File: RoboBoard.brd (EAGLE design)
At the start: 66 x 78.4 mm, 31 parts, among them IC2 L293D

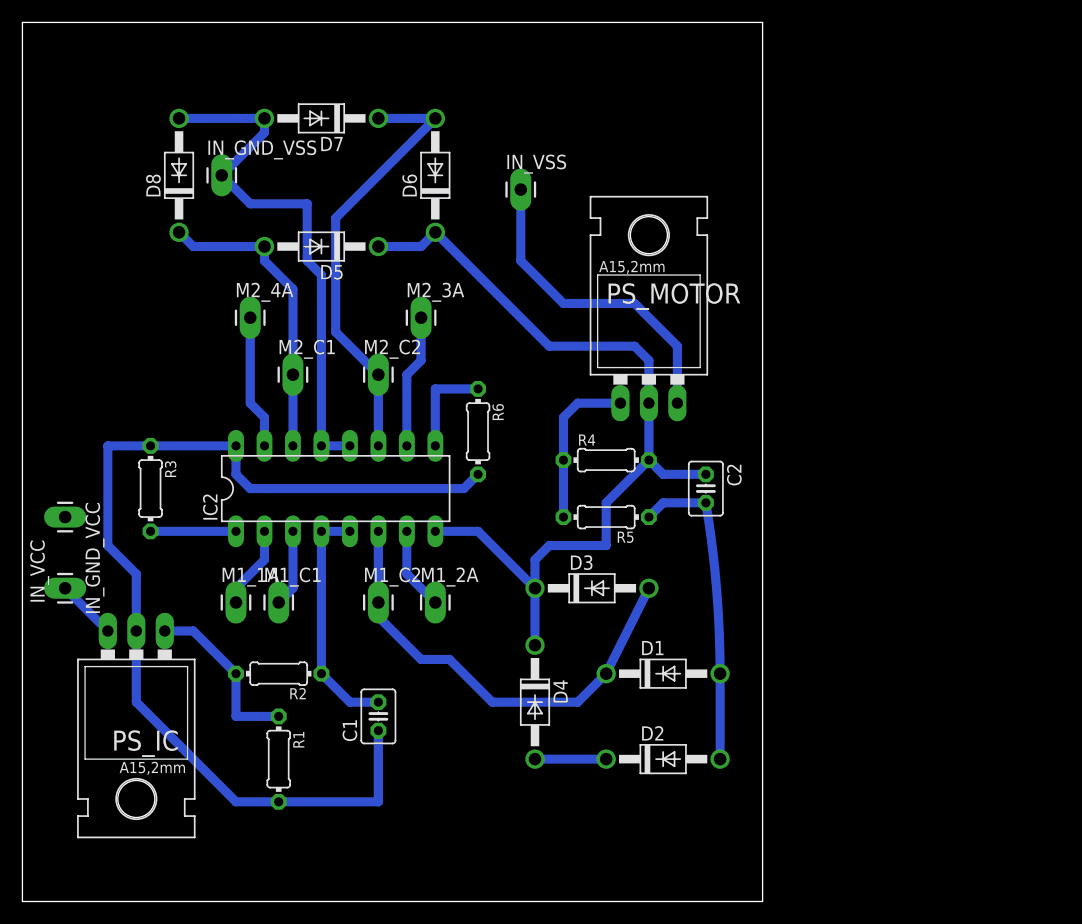
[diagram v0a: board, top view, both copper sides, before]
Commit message: fix:	Fixing board layout
Fixing the board layout
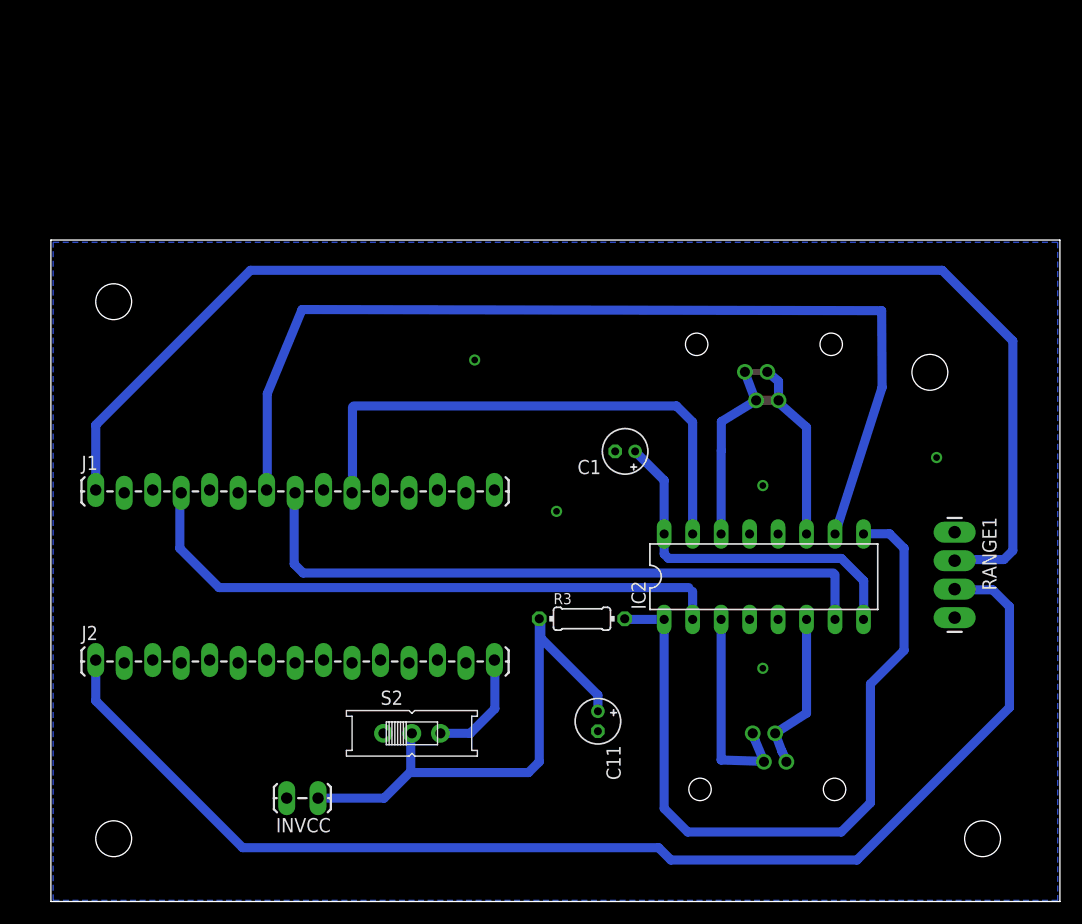
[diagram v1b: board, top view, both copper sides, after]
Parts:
- removed C2: 1u, resistor:C025-030X050
- removed D1, D2, D3, D4, D5, D6, D7, D8: 1N4004, diode:DO41-10
- removed IN_GND_VCC, IN_GND_VSS, IN_VCC, IN_VSS, M1_1A, M1_2A, M1_C1, M1_C2, M2_3A, M2_4A, M2_C1, M2_C2: (no value), SparkFun-Connectors:1X01_LONGPAD
- removed PS_IC, PS_MOTOR: (no value), v-reg:317TL
- removed R1, R4: 270, resistor:0204/7
- removed R2, R5: 820, resistor:0204/7
- removed R6: 10k, resistor:0204/7
- added C11: 0.1u, resistor:E1,8-4
- added INVCC: (no value), SparkFun-Connectors:1X02_LOCK_LONGPADS
- added J1, J2: (no value), SparkFun-Connectors:1X15_LOCK_LONGPADS
- added RANGE1: (no value), SparkFun-Connectors:1X04_LONGPADS
- added RJ1, RJ2: (no value), rj11:RJ11-4PIN
- added S2: (no value), adafruit:EG1218
- C1: value 0.1u -> 1u; device resistor:C025-030X050 -> resistor:E1,8-4
- moved R3 40.2 mm to (47.4, 25.2), turned to 0 degrees
- moved IC2 39.0 mm to (63.6, 29.0)
- moved C1 32.3 mm to (51.2, 40.1), turned to 180 degrees
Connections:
- removed net N$11: IC2.2, M1_1A.1
- removed net N$14: IC2.10, M2_3A.1
- removed net VSS: C2.1, D3.C, D4.C, D5.C, D6.C, IC2.8, PS_MOTOR.2, R4.2
- net GND: now also C1.-, C11.-, INVCC.2, J2.14, RANGE1.1; no longer C1.2, C2.2, D1.A, D2.A, D7.A, D8.A, IN_GND_VCC.1, IN_GND_VSS.1, R2.1, R5.1
- net N$1: now also IC2.3, RJ1.P$5; no longer IC2.1, R3.2
- net N$10: now also IC2.2, J1.4; no longer D6.A, D7.C, IC2.11, M2_C2.1
- net N$12: now also J1.1, RANGE1.2; no longer IC2.7, M1_2A.1
- net N$13: now also J2.15, S2.S; no longer IC2.15, M2_4A.1
- net N$2: now also IC2.6, RJ1.P$8; no longer PS_IC.1, R1.1, R2.2
- net N$3: now also IC2.11, RJ2.P$5, RJ2.P$6; no longer D2.C, D4.A, IC2.3, M1_C1.1
- net N$4: now also IC2.14, RJ2.P$7, RJ2.P$8; no longer D1.C, D3.A, IC2.6, M1_C2.1
- net N$5: now also IC2.15, J1.10; no longer IN_VSS.1, PS_MOTOR.3
- net N$6: now also J2.1, RANGE1.3; no longer IN_VCC.1, PS_IC.3
- net N$7: now also IC2.10, J1.7; no longer PS_MOTOR.1, R4.1, R5.2
- net N$8: now also IC2.1, R3.2; no longer R6.1
- net N$9: now also IC2.7, J1.8; no longer D5.A, D8.C, IC2.14, M2_C1.1
- net VCC: now also C1.+, C11.+, IC2.8, INVCC.1, RANGE1.4, S2.P; no longer C1.1, PS_IC.2, R1.2, R6.2
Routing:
- net N$12: track 7.40 -> 120.2 mm
- net N$6: track 5.39 -> 112.6 mm
- net GND: track 97.5 -> 0.00 mm, vias 0 -> 5
- net VSS: track 78.6 -> 0.00 mm
- net N$7: track 14.5 -> 89.7 mm
- net N$8: track 8.89 -> 68.9 mm
- net N$9: track 27.0 -> 59.0 mm
- net N$4: track 40.7 -> 15.7 mm, vias 0 -> 1
- net N$5: track 28.6 -> 48.6 mm
- net N$10: track 39.6 -> 54.8 mm
- net N$14: track 12.0 -> 0.00 mm
- net VCC: track 92.1 -> 80.2 mm
- net N$1: track 7.62 -> 19.2 mm
- net N$3: track 13.2 -> 22.6 mm, vias 0 -> 2
- net N$11: track 7.40 -> 0.00 mm
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- added copper zone on layer 16, net GND
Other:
- board size 66 x 78.4 mm -> 90 x 59 mm
